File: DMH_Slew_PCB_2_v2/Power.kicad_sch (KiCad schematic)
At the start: 29 parts, among them J0 Conn_01x01, J100 IDC_02x08, J200 IDC_02x05, J50 Conn_01x08_PinHeader, J51 Conn_01x08_PinHeader, J60 Conn_01x08_PinHeader, J61 Conn_01x08_PinHeader, U1 TL074, U10 LM4040LP-10, U11 LM4040LP-10, U2 TL074, U3 TL074, U4 TL074

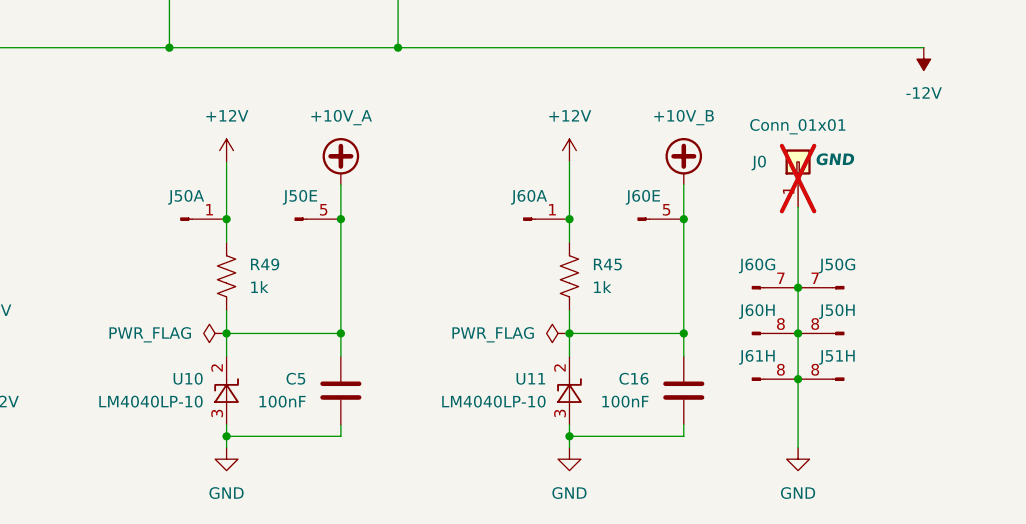
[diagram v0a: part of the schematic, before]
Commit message: Updated Log circuit
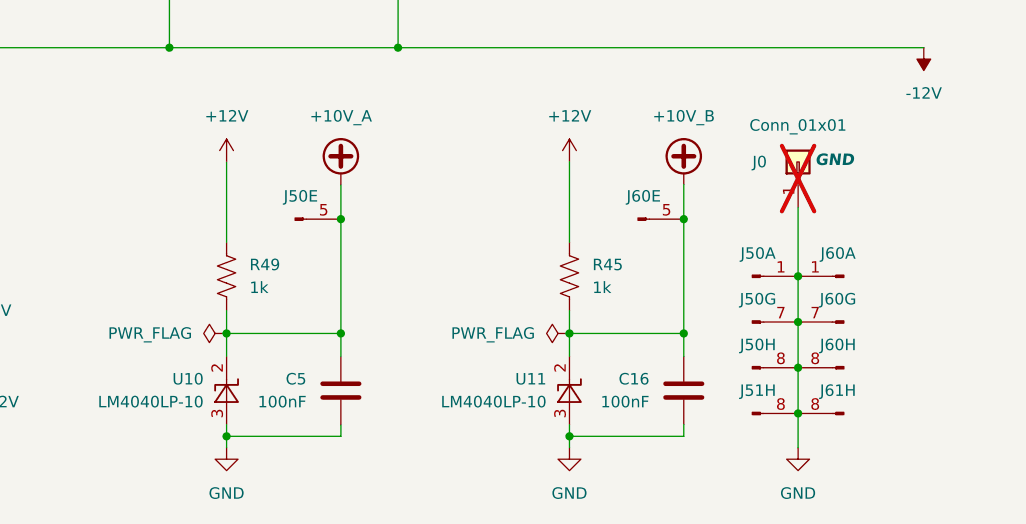
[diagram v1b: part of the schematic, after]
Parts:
- renumbered J60 to J50, J61 to J51, J50 to J60, J51 to J61
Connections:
- net +12V: no longer J50.1 (Pin_1), J60.1 (Pin_1)
- net GND: now also J50.1 (Pin_1), J60.1 (Pin_1)
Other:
- moved on the sheet: J50G, J50H, J51H, J60G, J60H, J61H
